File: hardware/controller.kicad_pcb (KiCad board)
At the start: 4 copper layers, 29 x 74 mm, 66 parts, among them J11 UART, J12 JST 2.0 BATT, J9 Chip Enable, P1 USB_C_Plug_USB2.0, U1 THB001P, U5 ESP32-H2-MINI-1, U6 AP2204, U7 MCP73833

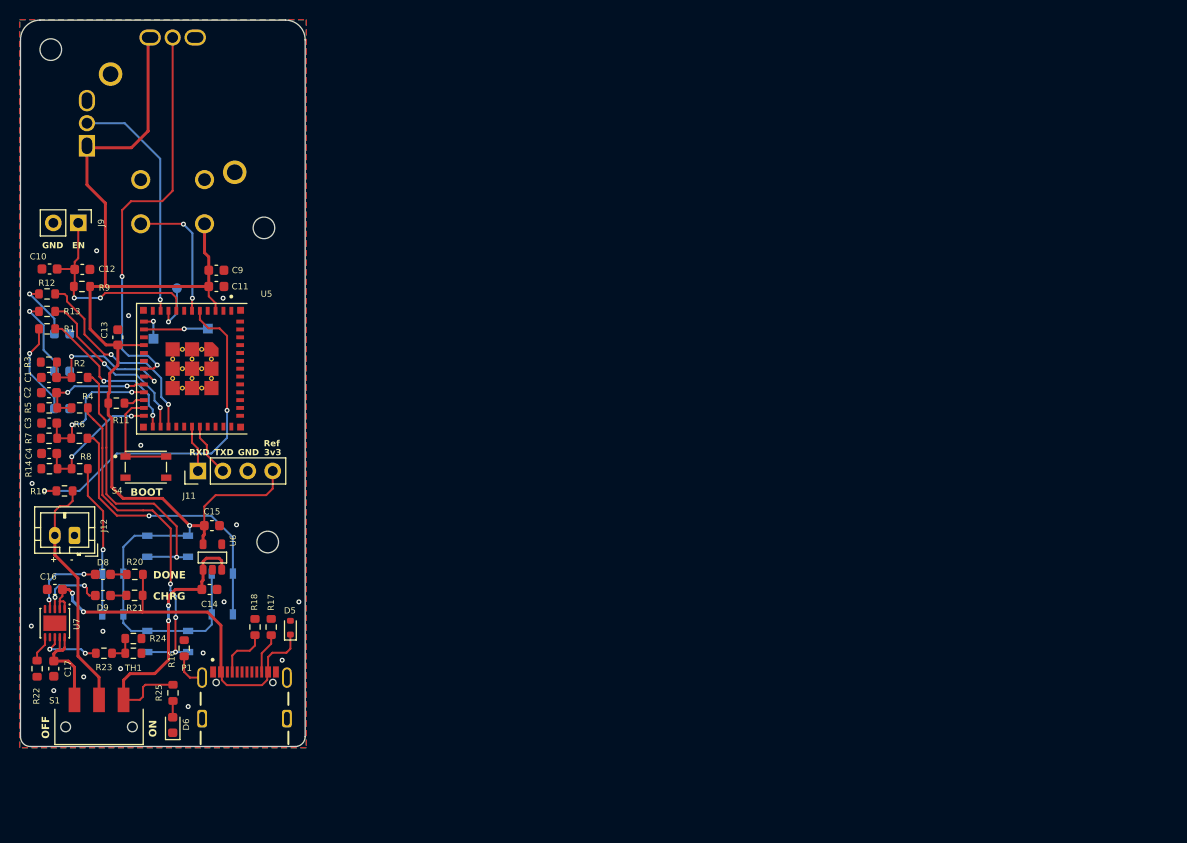
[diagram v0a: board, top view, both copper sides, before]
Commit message: hardware v1.0
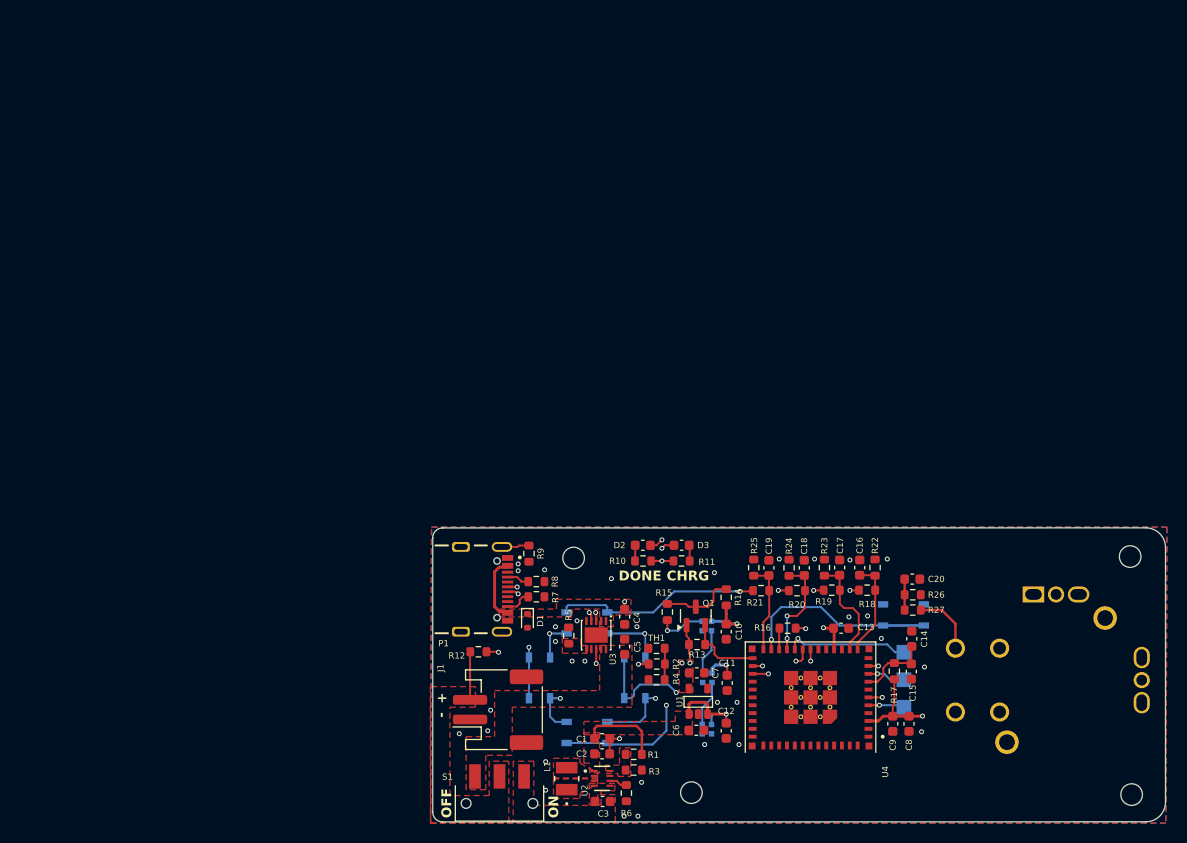
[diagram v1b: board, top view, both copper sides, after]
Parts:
- removed the C14 at (77.2, 87.0)
- removed the C15 at (77.5, 80.5)
- removed the C16 at (61.5, 87.0)
- removed the C17 at (61.4, 95.1)
- removed D5: TPD1E10B06DPYR, Diode_SMD:D_SOD-523
- removed D6: PWLED, Diode_SMD:D_0603_1608Metric
- removed D8, D9: LED, Capacitor_SMD:C_0603_1608Metric
- removed J11: UART, Connector_PinHeader_2.54mm:PinHeader_1x04_P2.54mm_Vertical
- removed J12: JST 2.0 BATT, Connector_JST:JST_PH_B2B-PH-K_1x02_P2.00mm_Vertical
- removed J9: Chip Enable, Connector_PinHeader_2.54mm:PinHeader_1x02_P2.54mm_Vertical
- removed the R16 at (74.7, 93.0)
- removed the R17 at (83.5, 90.8)
- removed the R18 at (81.9, 90.8)
- removed the R20 at (69.6, 85.5)
- removed the R21 at (69.6, 87.6)
- removed the R22 at (59.7, 95.1)
- removed the R23 at (66.5, 93.5)
- removed the R24 at (69.5, 92.0)
- removed the R25 at (73.5, 97.5)
- removed the REF** at (83.2, 56.3)
- removed the S4 at (70.8, 74.5)
- removed the TP1 at (71.6, 61.5)
- removed TP2: 0_IN2, TestPoint:TestPoint_Pad_1.0x1.0mm
- removed U6: AP2204, kicad_reformed_custom_IC:AP2204
- removed U7: MCP73833, kicad_reformed_custom_IC:SON50P300X300X100-11N
- added C1: 10uF, Capacitor_SMD:C_0603_1608Metric, F.Cu at (117.2, 102.2)
- added C10: 0.1uF, Capacitor_SMD:C_0603_1608Metric, F.Cu at (129.9, 91.3)
- added C11: 0.1uF, Capacitor_SMD:C_0603_1608Metric, F.Cu at (130.0, 96.5)
- added C12: 0.1uF, Capacitor_SMD:C_0603_1608Metric, F.Cu at (129.9, 101.4)
- added C2: 10uF, Capacitor_SMD:C_0603_1608Metric, F.Cu at (117.2, 103.8)
- added C20: 1uF, Capacitor_SMD:C_0603_1608Metric, F.Cu at (148.8, 86.0)
- added C3: 10uF, Capacitor_SMD:C_0603_1608Metric, F.Cu at (117.3, 108.6)
- added C4: 10uF, Capacitor_SMD:C_0603_1608Metric, F.Cu at (119.5, 89.8)
- added C5: 47uF, Capacitor_SMD:C_0603_1608Metric, F.Cu at (119.5, 92.8)
- added C6: 10uF, Capacitor_SMD:C_0603_1608Metric, F.Cu at (126.8, 101.3)
- added C7: 10uF, Capacitor_SMD:C_0603_1608Metric, F.Cu at (126.9, 95.5)
- added J1: JST 2.0 BATT, Connector_JST:JST_PH_S2B-PH-SM4-TB_1x02-1MP_P2.00mm_Horizontal, F.Cu at (106.7, 99.2)
- added L1: 1uH, custom_IC:RES_CIGT252010, F.Cu at (113.7, 106.3)
- added LED1: IN-PI15TAT5R5G5B, custom_IC:IN-PI15_INL, B.Cu at (127.9, 90.7)
- added LED2: IN-PI15TAT5R5G5B, custom_IC:IN-PI15_INL, B.Cu at (128.0, 96.0)
- added LED3: IN-PI15TAT5R5G5B, custom_IC:IN-PI15_INL, B.Cu at (127.9, 101.2)
- added Q1: BSS138, Package_TO_SOT_SMD:SOT-23, F.Cu at (126.8, 89.7)
- added R11: 330, Resistor_SMD:R_0603_1608Metric, F.Cu at (125.3, 84.1)
- added R14: 10K, Resistor_SMD:R_0603_1608Metric, F.Cu at (129.9, 87.8)
- added R15: 470, Resistor_SMD:R_0603_1608Metric, F.Cu at (123.9, 89.3)
- added R2: 1.43K, Resistor_SMD:R_0603_1608Metric, F.Cu at (122.8, 94.6)
- added R26: 100K, Resistor_SMD:R_0603_1608Metric, F.Cu at (148.9, 87.5)
- added R27: 10K, Resistor_SMD:R_0603_1608Metric, F.Cu at (148.9, 89.1)
- added R3: 91, Resistor_SMD:R_0603_1608Metric, F.Cu at (120.5, 105.4)
- added R4: 75K, Resistor_SMD:R_0603_1608Metric, F.Cu at (122.8, 96.2)
- added R5: 5K1, Resistor_SMD:R_0603_1608Metric, F.Cu at (113.8, 91.7)
- added R6: 10K, Resistor_SMD:R_0603_1608Metric, F.Cu at (119.7, 107.8)
- added R7: 5K1, Resistor_SMD:R_0603_1608Metric, F.Cu at (110.5, 87.8)
- added R8: 5K1, Resistor_SMD:R_0603_1608Metric, F.Cu at (110.5, 86.2)
- added R9: 1M, Resistor_SMD:R_0603_1608Metric, F.Cu at (109.8, 83.3)
- added REF**: MountingHole_2.2mm_M2, MountingHole:MountingHole_2.2mm_M2, F.Cu at (114.3, 83.8)
- added S6: TL4100AF240QG_, kicad_reformed_custom_IC:SW_PTS810_SJM_250_SMTR_LFS, B.Cu at (147.9, 89.6)
- added TP3: TP, TestPoint:TestPoint_Pad_1.5x1.5mm, B.Cu at (148.0, 99.0)
- added TP5: TP, TestPoint:TestPoint_Pad_1.5x1.5mm, B.Cu at (148.0, 93.4)
- added U1: AP2205, kicad_reformed_custom_IC:AP2204, F.Cu at (127.0, 98.4)
- added U2: TPS631000DRLR, custom_IC:TPS631000DRLR_TEX, F.Cu at (117.3, 106.3)
- added U3: MCP73833, kicad_reformed_custom_IC:SON50P300X300X100-11N, F.Cu at (116.7, 91.7)
- C14: renamed from C10; value 1uF 25V -> 1uF
- C16: renamed from C1; value 1uF 25V -> 1uF
- C17: renamed from C2; value 1uF 25V -> 1uF
- C18: renamed from C3; value 1uF 25V -> 1uF
- C19: renamed from C4; value 1uF 25V -> 1uF
- D1: value LED -> TPD1E10B06DPYR; footprint Capacitor_SMD:C_0603_1608Metric -> Diode_SMD:D_SOD-523; moved to F.Cu
- D2: value LED -> LED_GREEN; moved to F.Cu
- D3: value LED -> LED_RED; moved to F.Cu
- R1: value 200 -> 806
- R10: value 10k -> 330
- R12, R13: value 200 -> 10K
- R16: renamed from R11; value 10k -> 10K
- R17: renamed from R9; value 10k -> 10K
- R18: renamed from R2; value 10k -> 10K
- R19: renamed from R4; value 10k -> 10K
- R20: renamed from R6; value 10k -> 10K
- R21: renamed from R8; value 10k -> 10K
- R22: renamed from R3; value 100k -> 100K
- R23: renamed from R5; value 100k -> 100K
- R24: renamed from R7; value 100k -> 100K
- R25: renamed from R14; value 100k -> 100K
- TH1: value TH 10k -> TH 10K
- TP1: renamed from TP3; footprint TestPoint:TestPoint_Pad_D1.0mm -> TestPoint:TestPoint_Pad_1.5x1.5mm
- moved REF** 121.5 mm to (171.1, 83.7), turned to -90 degrees
- moved U5 106.4 mm to (163.5, 96.2), turned to 90 degrees
- moved REF** 105.6 mm to (171.2, 107.9), turned to -90 degrees
- moved C14 95.6 mm to (148.8, 92.0), turned to 90 degrees
- moved C15 93.9 mm to (148.8, 95.4), turned to -90 degrees
- moved R17 91.6 mm to (147.0, 95.3), turned to 90 degrees
- moved R22 86.7 mm to (145.1, 84.8), turned to 90 degrees
- moved C16 84.8 mm to (143.5, 84.8), turned to 90 degrees
- moved C8 84.3 mm to (148.5, 100.7), turned to -90 degrees
- moved TP1 84.1 mm to (148.0, 96.2), turned to 90 degrees
- moved R18 83.1 mm to (144.2, 87.1), turned to 180 degrees
- moved C17 82.5 mm to (141.4, 84.8), turned to 90 degrees
- moved C9 82.1 mm to (146.9, 100.7), turned to -90 degrees
- moved R23 80.6 mm to (139.9, 84.8), turned to 90 degrees
- moved C13 79.4 mm to (141.6, 91.0), turned to 0 degrees
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- renumbered C12 to C15, C9 to C8, C11 to C9, S5 to S4, S6 to S5, U5 to U4, U1 to U5
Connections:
- D1 pad 1: GND -> +5VD
- D1 pad 2: Net-(D1-A) -> GND
- D2 pad 1: GND -> /STAT2_DONE
- D3 pad 1: GND -> /STAT1_CHARGING
- P1 pad A4: +5V -> +5VD
- P1 pad A6: unconnected-(P1-D+-PadA6) -> /USB_D+
- P1 pad A7: unconnected-(P1-D--PadA7) -> /USB_D-
- P1 pad A9: +5V -> +5VD
- R1 pad 1: Net-(D3-A) -> +5V
- R1 pad 2: Net-(U5-IO25) -> Net-(U2-FB)
- R10 pad 1: LIPO+ -> +5VD
- R10 pad 2: /ADC_BATT -> Net-(D2-A)
- R12 pad 1: Net-(D1-A) -> LIPO+
- R12 pad 2: Net-(U5-IO27) -> /ADC_BATT
- R13 pad 1: Net-(D2-A) -> Net-(Q1-S)
- R13 pad 2: Net-(U5-IO26) -> +3V3
- S1 pad 3: /raw_voltage -> RAW
- U4 pad 12: Net-(U5-IO13) -> /SW_A
- U4 pad 13: Net-(U5-IO14) -> /SW_B
- U4 pad 19: /SW_A -> /ADC_BATT
- U4 pad 20: /SW_B -> Net-(U4-IO10)
- U4 pad 25: Net-(U5-IO25) -> Net-(Q1-S)
- U4 pad 26: Net-(U5-IO26) -> /USB_D-
- U4 pad 27: Net-(U5-IO27) -> /USB_D+
- U4 pad 30: /U0RXD -> unconnected-(U4-RXD0-Pad30)
- U4 pad 31: /U0TXD -> unconnected-(U4-TXD0-Pad31)
- U4 pad 5: /ADC_BATT -> Net-(U4-IO2)
- U5 pad B: (no net) -> +3V3
- U5 pad C: +3V3 -> (no net)
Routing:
- net +3V3: track 133.5 -> 40.1 mm, vias 1 -> 9
- net /USB_D+: track 0.00 -> 32.6 mm, vias 0 -> 2
- net /USB_D-: track 0.00 -> 30.5 mm, vias 0 -> 2
- net /raw_voltage: track 29.8 -> 0.00 mm, vias 2 -> 0
- net Net-(U5-IO27): track 20.8 -> 0.00 mm, vias 2 -> 0
- net GND: track 23.3 -> 2.55 mm, vias 16 -> 33
- net LIPO+: track 24.4 -> 4.91 mm
- net Net-(U5-IO26): track 18.0 -> 0.00 mm, vias 2 -> 0
- net Net-(U5-IO25): track 16.4 -> 0.00 mm, vias 2 -> 0
- net +5VD: track 0.00 -> 16.2 mm, vias 0 -> 2
- net /STAT2_DONE: track 0.00 -> 14.5 mm, vias 0 -> 2
- net /CP_EN: track 21.8 -> 7.46 mm, vias 2 -> 0
- net /STAT1_CHARGING: track 0.00 -> 13.2 mm, vias 0 -> 2
- net Net-(U4-IO10): track 0.00 -> 12.6 mm, vias 0 -> 1
- net /CHRGR+: track 10.2 -> 0.00 mm
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- added copper zone on F.Cu, net +3V3
- added copper zone on In1.Cu, net +3V3
- added copper zone on F.Cu, net +5V
- added copper zone on F.Cu, net +5VD
- added copper zone on F.Cu, net /CHRGR+
- added copper zone on In2.Cu, net GND
- added copper zone on F.Cu, net LIPO+
- added copper zone on F.Cu, net Net-(U2-FB)
- added copper zone on F.Cu, net Net-(U2-LX1)
- added copper zone on F.Cu, net Net-(U2-LX2)
- added copper zone on F.Cu, net Net-(U3-PROG)
- added copper zone on F.Cu, net RAW
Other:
- board size 29 x 74 mm -> 74.7 x 30 mm
- board text added: "Batt"
- board text added: "StuckAtPrototype"
- board text added: "Thumbtroller V1.0"
- board text removed: "3v3"
- board text removed: "EN"
- board text removed: "GND"
- board text removed: "Low Batt"
- board text removed: "RXD"
- board text removed: "Ref"
- board text removed: "StuckAtPrototype DMsensors"
- board text removed: "TXD"
- board text removed: "Thumbtroller V0.2"
